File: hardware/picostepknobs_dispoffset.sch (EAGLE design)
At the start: 57 parts, among them J1 AUDIO-JACK-TRRS, J2 AUDIO-JACK-TRRS, P1 10k, P2 10k, P3 10k, P4 10k, P5 10k, P6 10k, P7 10k, P8 10k, U1 RASPBERRY_PICOSMD-TH, U2 4051D, U3 H11L1MS

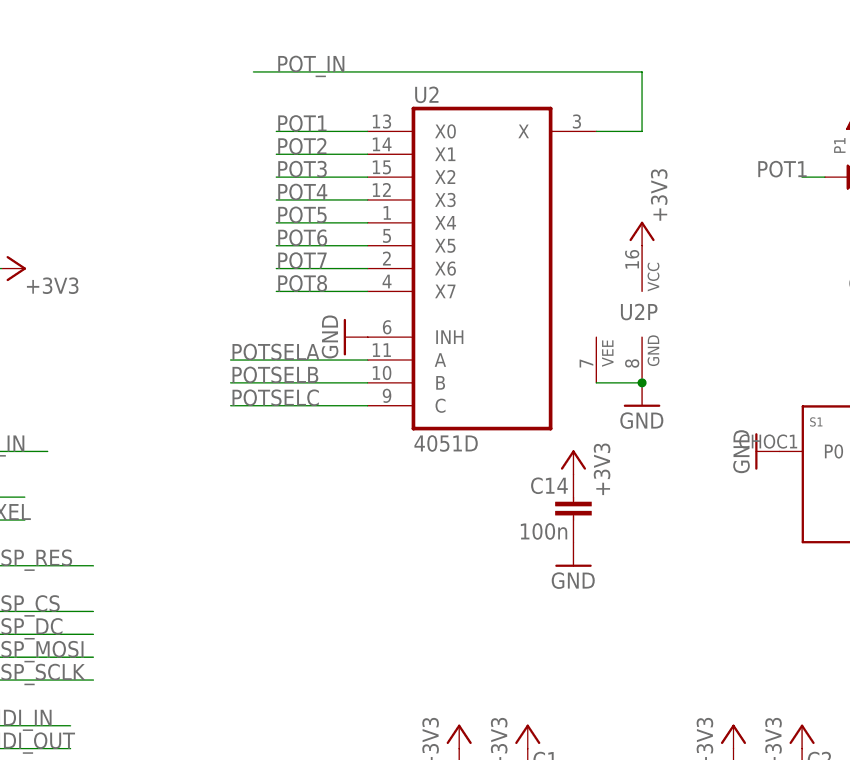
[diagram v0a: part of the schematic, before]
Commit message: it is working a little
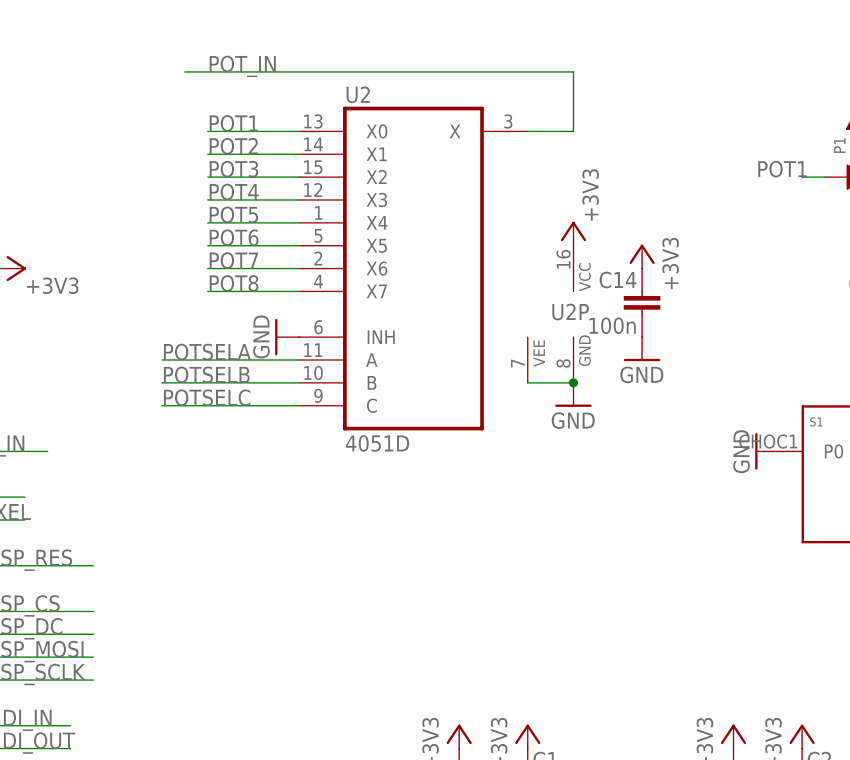
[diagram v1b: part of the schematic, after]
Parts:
- LED1, LED10, LED11, LED12, LED2, LED3, LED4, LED5, LED6, LED7, LED8, LED9: value WS2812B3535 -> WS2812B5050; device todstuff2023:WS2812B3535 -> todstuff2023:WS2812B5050
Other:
- moved on the sheet: C14, U2, U2P
